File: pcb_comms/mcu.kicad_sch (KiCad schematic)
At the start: 25 parts, among them U2 STM32WLE5CCU6, Y1 G43270018, Y3 32MHz

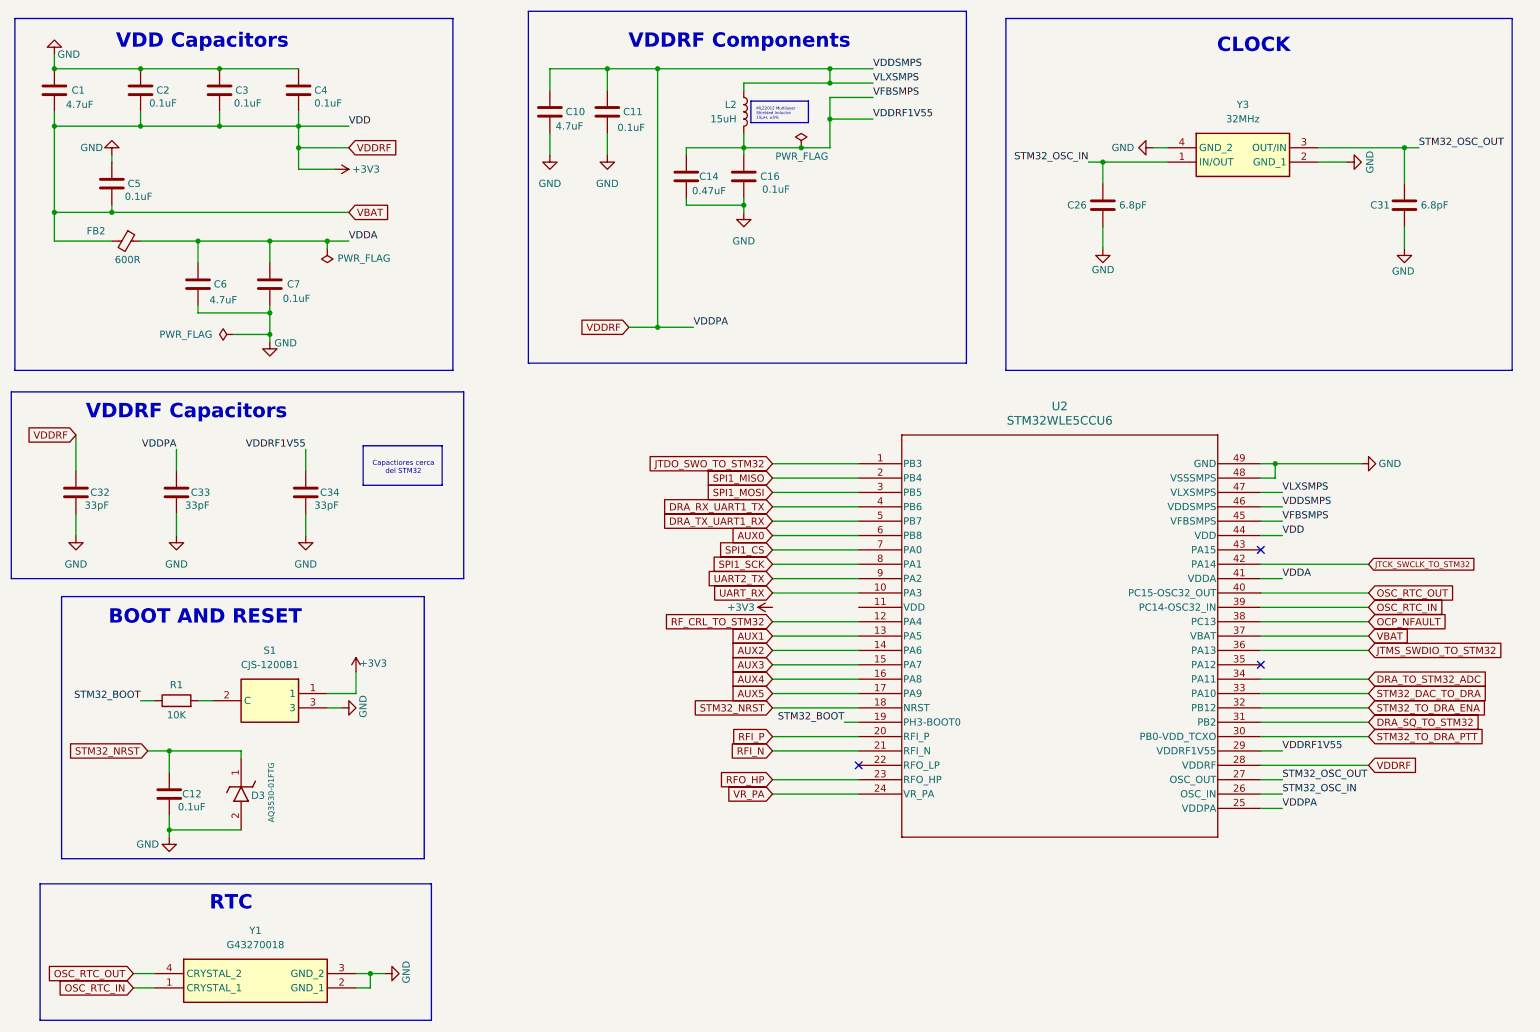
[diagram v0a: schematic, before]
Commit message: Update schematic
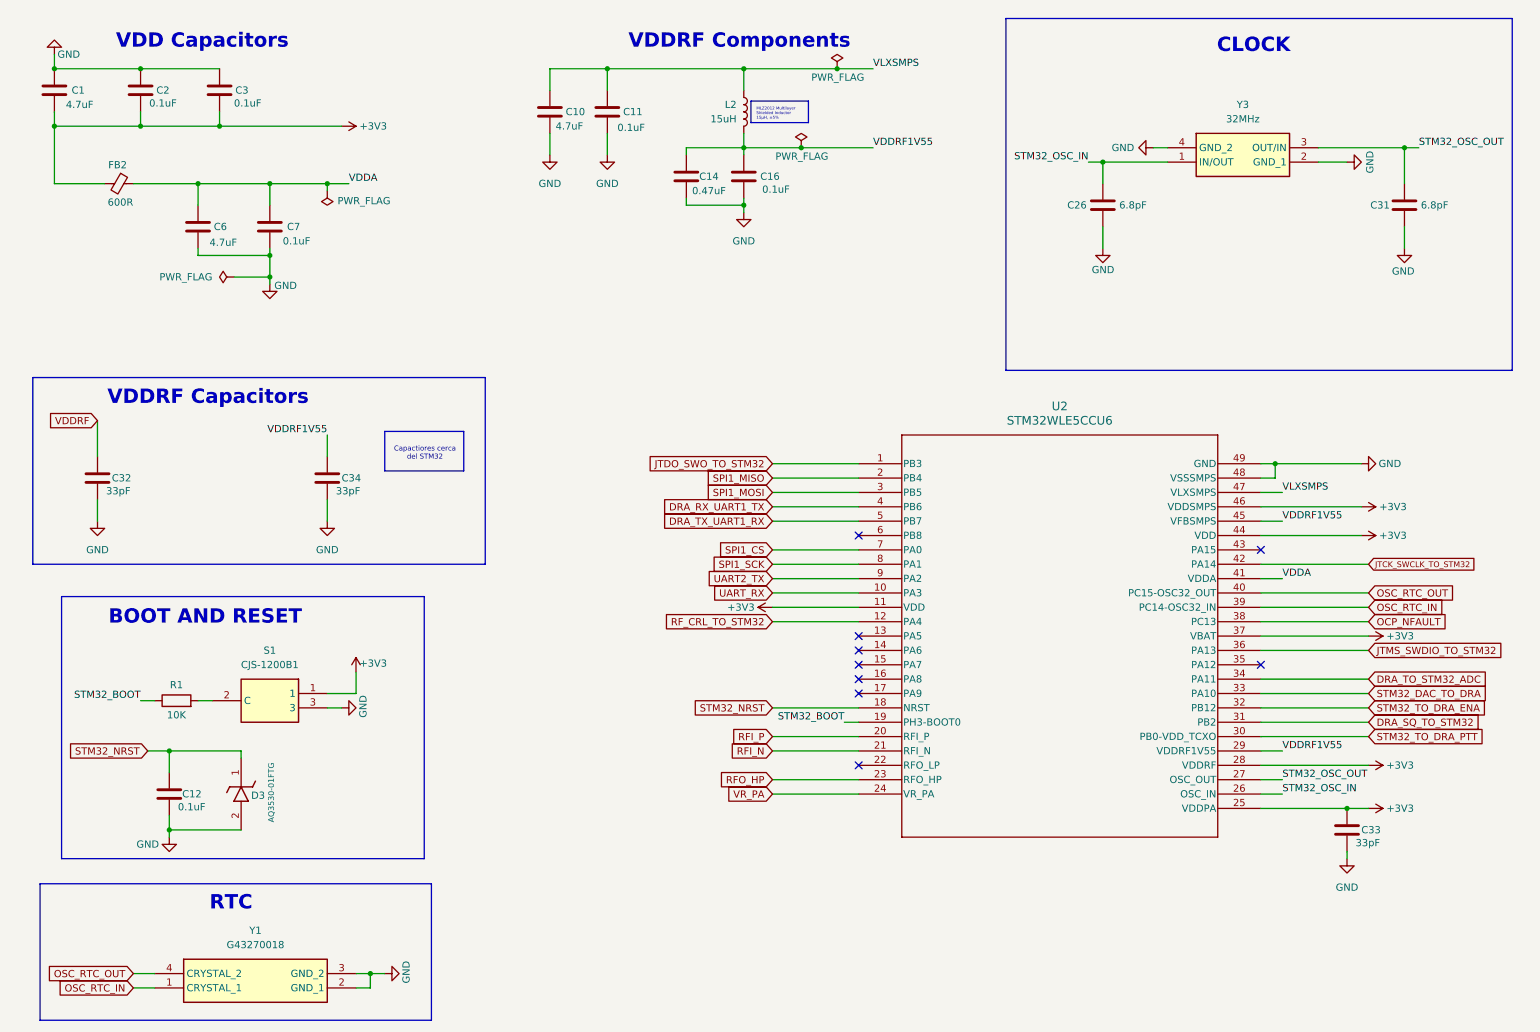
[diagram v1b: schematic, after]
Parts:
- removed C4, C5: 0.1uF, Capacitor_SMD:C_0805_2012Metric_Pad1.18x1.45mm_HandSolder, symbol Device:C
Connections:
- net +3V3: now also U2.11 (VDD); no longer C10.1, C11.1, C32.1, L2.1, U2.47 (VLXSMPS)
- net AUX0: no longer names the net of U2.6 (PB8)
- net AUX1: no longer names the net of U2.13 (PA5)
- net AUX2: no longer names the net of U2.14 (PA6)
- net AUX3: no longer names the net of U2.15 (PA7)
- net AUX4: no longer names the net of U2.16 (PA8)
- net AUX5: no longer names the net of U2.17 (PA9)
- new net VDDRF: C32.1
- new net VLXSMPS: C10.1, C11.1, L2.1, U2.47 (VLXSMPS)
- no-connect marks 3 -> 9
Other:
- moved on the sheet: C32, C33, C34, C6, C7, FB2
